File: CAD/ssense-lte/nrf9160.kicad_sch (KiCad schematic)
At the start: 43 parts, among them J1 HIROSE ELECTRIC U.FL-R-SMT-1, J3 693043020611, J4 HIROSE ELECTRIC U.FL-R-SMT-1, J6 JLINK, SW1 KMR223NGLFG, U5 nRF9160-SICA, U8 USBLC6-4SC6, U9 TPS22917DBV

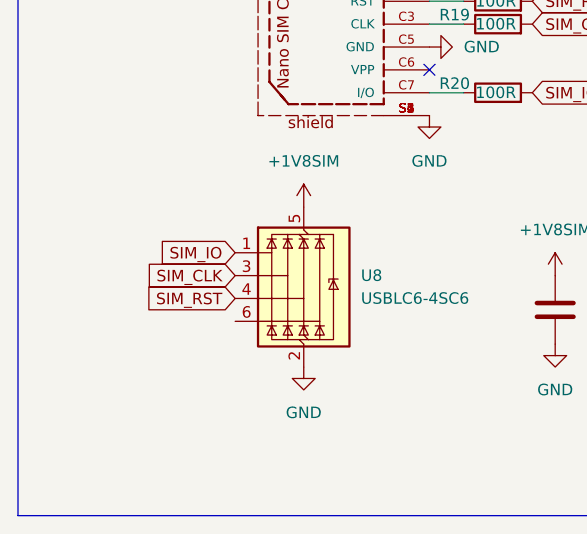
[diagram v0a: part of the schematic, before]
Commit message: Backup commit
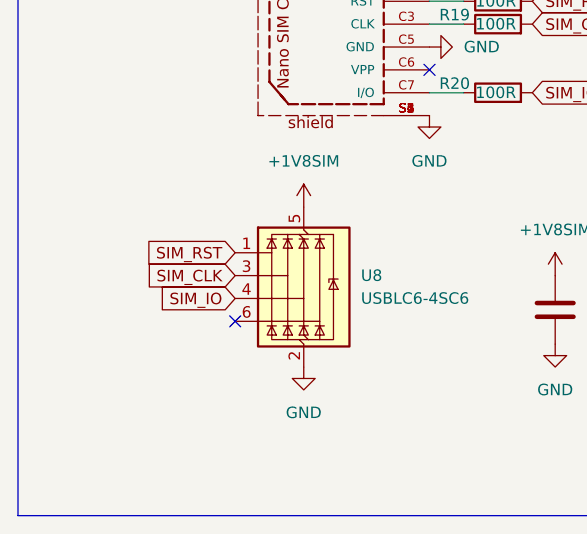
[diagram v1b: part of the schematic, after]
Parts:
- R17, R18, R19, R20, R29: footprint Resistor_SMD:R_0603_1608Metric -> Resistor_SMD:R_0402_1005Metric
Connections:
- net SIM_IO: now also U8.4 (I/O3); no longer U8.1 (I/O1)
- net SIM_RST: now also U8.1 (I/O1); no longer U8.4 (I/O3)
- no-connect marks 18 -> 19
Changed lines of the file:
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@@
 	)
 	(no_connect
+		(at 38.1 175.26)
+	)
+	(no_connect
 		(at 228.6 92.71)
 	)
@@
 	(global_label "SIM_RST"
 		(shape input)
-		(at 38.1 172.72 180)
+		(at 38.1 167.64 180)
 		(fields_autoplaced yes)
 		(effects
@@
 		)
 		(property "Intersheetrefs" "${INTERSHEET_REFS}"
-			(at 27.4344 172.72 0)
+			(at 28.9462 167.64 0)
 			(effects
 				(font
@@
 	(global_label "SIM_IO"
 		(shape input)
-		(at 38.1 167.64 180)
+		(at 38.1 172.72 180)
 		(fields_autoplaced yes)
 		(effects
@@
 		)
 		(property "Intersheetrefs" "${INTERSHEET_REFS}"
-			(at 28.9462 167.64 0)
+			(at 27.4344 172.72 0)
 			(effects
 				(font
@@
 			)
 		)
-		(property "Footprint" "Resistor_SMD:R_0603_1608Metric"
+		(property "Footprint" "Resistor_SMD:R_0402_1005Metric"
 			(at 67.31 151.638 90)
 			(effects
@@
 			)
 		)
-		(property "Footprint" "Resistor_SMD:R_0603_1608Metric"
+		(property "Footprint" "Resistor_SMD:R_0402_1005Metric"
 			(at 254 36.322 90)
 			(effects
@@
 			)
 		)
-		(property "Footprint" "Resistor_SMD:R_0603_1608Metric"
+		(property "Footprint" "Resistor_SMD:R_0402_1005Metric"
 			(at 67.31 141.478 90)
 			(effects
@@
 			)
 		)
-		(property "Footprint" "Resistor_SMD:R_0603_1608Metric"
+		(property "Footprint" "Resistor_SMD:R_0402_1005Metric"
 			(at 67.31 144.018 90)
 			(effects
@@
 			)
 		)
-		(property "Footprint" "Resistor_SMD:R_0603_1608Metric"
+		(property "Footprint" "Resistor_SMD:R_0402_1005Metric"
 			(at 208.788 99.06 90)
 			(effects
